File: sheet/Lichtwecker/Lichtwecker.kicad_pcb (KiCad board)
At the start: 2 copper layers, 3 parts

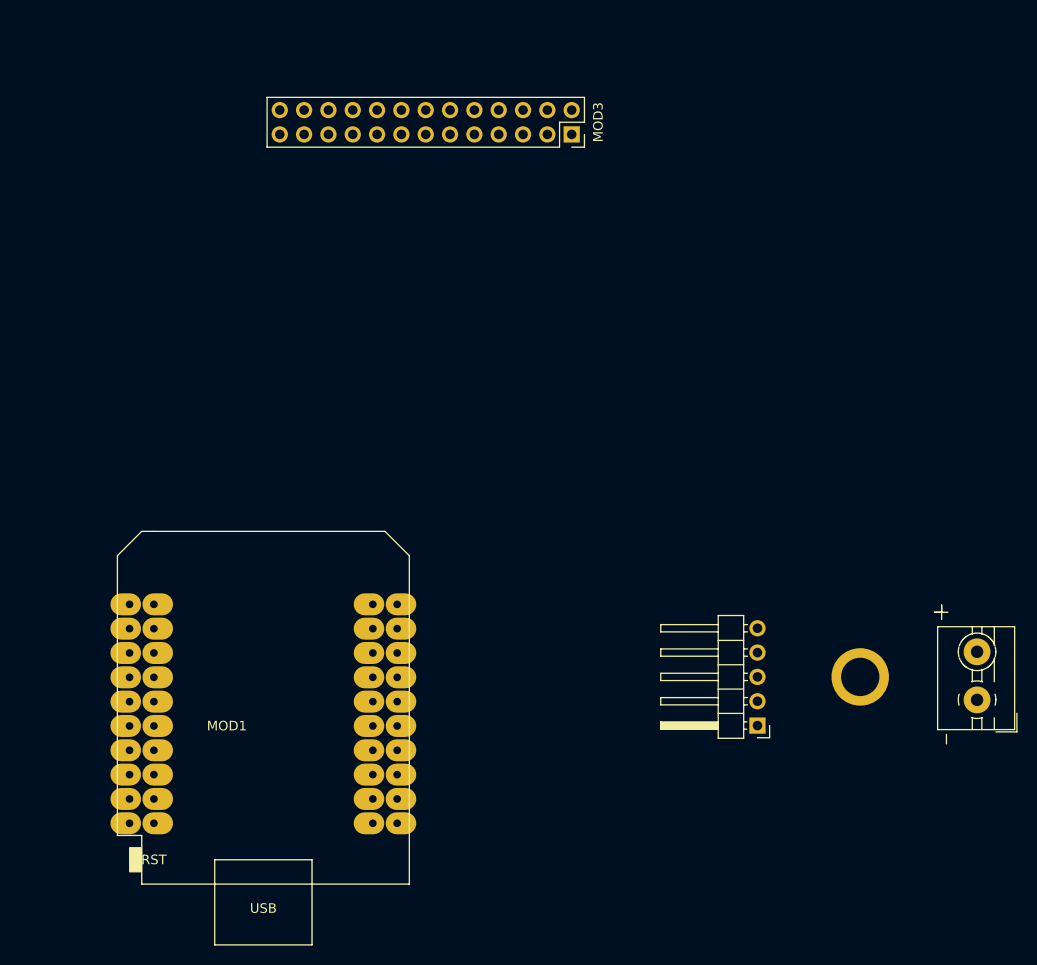
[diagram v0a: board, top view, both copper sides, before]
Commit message: OPT: Schaltplan angepasst
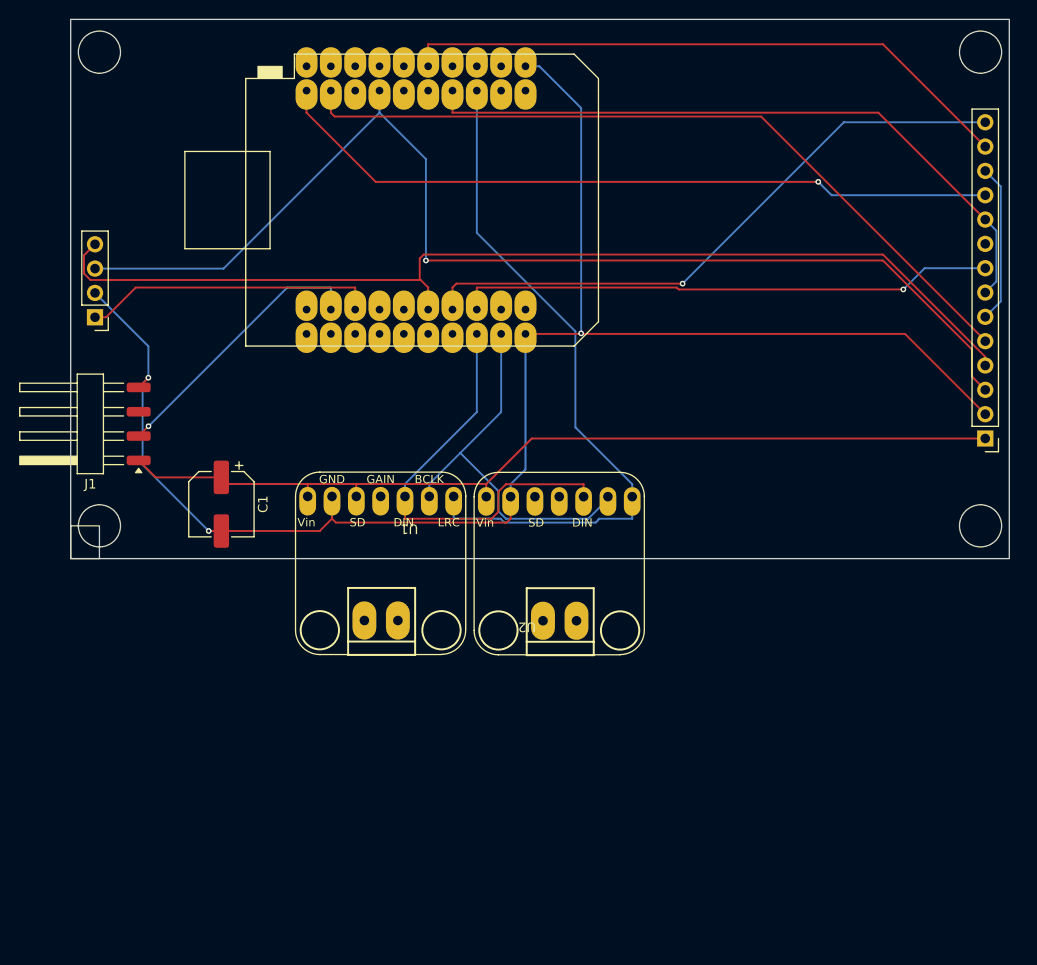
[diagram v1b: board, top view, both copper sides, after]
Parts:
- removed MOD2: ~, 01_MyLib:Modul MAX6675 K-typ Thermoelement
- removed MOD3: ~, Connector_PinSocket_2.54mm:PinSocket_2x13_P2.54mm_Vertical
- added C1: 1000uF, Capacitor_SMD:CP_Elec_6.3x5.9, F.Cu at (104.6, 75.2)
- added J1: Conn_01x04_Pin, Connector_Harwin:Harwin_M20-89004xx_1x04_P2.54mm_Horizontal, F.Cu at (90.5, 66.8)
- added U1: adafruit-MAX98357, adafruit-MAX98357:adafruit-MAX98357, F.Cu at (121.2, 81.3)
- added U2: adafruit-MAX98357, adafruit-MAX98357:adafruit-MAX98357, F.Cu at (139.8, 81.3)
- added U3: ~, 01_MyLib:3.5_TFT_Touch_SPI_Display, F.Cu at (88.9, 80.9)
- moved MOD1 56.0 mm to (125.0, 43.4), turned to -90 degrees
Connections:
- MOD1 pad 10: Net-(MOD1-IO_19/D6) -> unconnected-(MOD1-IO_19/D6-Pad10)
- MOD1 pad 11: unconnected-(MOD1-IO_34-Pad11) -> Net-(MOD1-IO_34)
- MOD1 pad 12: Net-(MOD1-IO_23/D7) -> unconnected-(MOD1-IO_23/D7-Pad12)
- MOD1 pad 17: Net-(MOD1-IO_09/SD2) -> unconnected-(MOD1-IO_09/SD2-Pad17)
- MOD1 pad 18: unconnected-(MOD1-IO_13/TCK-Pad18) -> Net-(MOD1-IO_13/TCK)
- MOD1 pad 20: unconnected-(MOD1-IO_10/SD3-Pad20) -> Net-(MOD1-IO_10/SD3)
- MOD1 pad 24: unconnected-(MOD1-IO_27-Pad24) -> Net-(MOD1-IO_27)
- MOD1 pad 25: unconnected-(MOD1-IO_22/D1/SCL-Pad25) -> Net-(MOD1-IO_22/D1/SCL)
- MOD1 pad 26: unconnected-(MOD1-IO_25-Pad26) -> Net-(MOD1-IO_25)
- MOD1 pad 27: unconnected-(MOD1-IO_21/D2/SDA-Pad27) -> Net-(MOD1-IO_21/D2/SDA)
- MOD1 pad 29: unconnected-(MOD1-IO_17/D3-Pad29) -> Net-(MOD1-IO_17/D3)
- MOD1 pad 32: Net-(MOD1-IO_04) -> unconnected-(MOD1-IO_04-Pad32)
- MOD1 pad 34: Net-(MOD1-IO_00) -> unconnected-(MOD1-IO_00-Pad34)
- MOD1 pad 36: Net-(MOD1-IO_02) -> unconnected-(MOD1-IO_02-Pad36)
- MOD1 pad 37: unconnected-(MOD1-TD0-Pad37) -> RGB_SDA
- MOD1 pad 6: unconnected-(MOD1-IO_26/D0-Pad6) -> Net-(MOD1-IO_26/D0)
- MOD1 pad 9: unconnected-(MOD1-IO_33-Pad9) -> Net-(MOD1-IO_33)
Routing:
- net GND: track 0.00 -> 169.0 mm, vias 0 -> 3
- net +5V: track 0.00 -> 126.1 mm
- net Net-(MOD1-IO_05/D8): track 0.00 -> 121.8 mm, vias 0 -> 1
- net Net-(MOD1-IO_17/D3): track 0.00 -> 109.2 mm
- net Net-(MOD1-IO_13/TCK): track 0.00 -> 80.5 mm
- net Net-(MOD1-IO_10/SD3): track 0.00 -> 76.7 mm, vias 0 -> 1
- net Net-(MOD1-IO_26/D0): track 0.00 -> 72.7 mm
- net Net-(MOD1-IO_18/D5): track 0.00 -> 71.1 mm
- net Net-(MOD1-IO_21/D2/SDA): track 0.00 -> 65.1 mm, vias 0 -> 1
- net Net-(MOD1-IO_33): track 0.00 -> 64.9 mm
- net Net-(MOD1-IO_22/D1/SCL): track 0.00 -> 56.4 mm, vias 0 -> 1
- net Net-(MOD1-IO_25): track 0.00 -> 45.1 mm
- net Net-(MOD1-IO_27): track 0.00 -> 40.7 mm
- net RGB_SDA: track 0.00 -> 28.8 mm, vias 0 -> 1
- net Net-(MOD1-IO_34): track 0.00 -> 16.6 mm
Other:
- board outline added: 98 x 56.3 mm
- board text added: "BCLK"
